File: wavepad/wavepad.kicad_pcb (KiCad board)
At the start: 2 copper layers, 18 parts, among them SW1 SW_Push, SW2 SW_Push, SW3 SW_Push, SW4 SW_Push, SW5 SW_Push, SW6 SW_Push, SW7 SW_Push, SW8 SW_Push, U1 Seeed Studio XIAO SAMD21

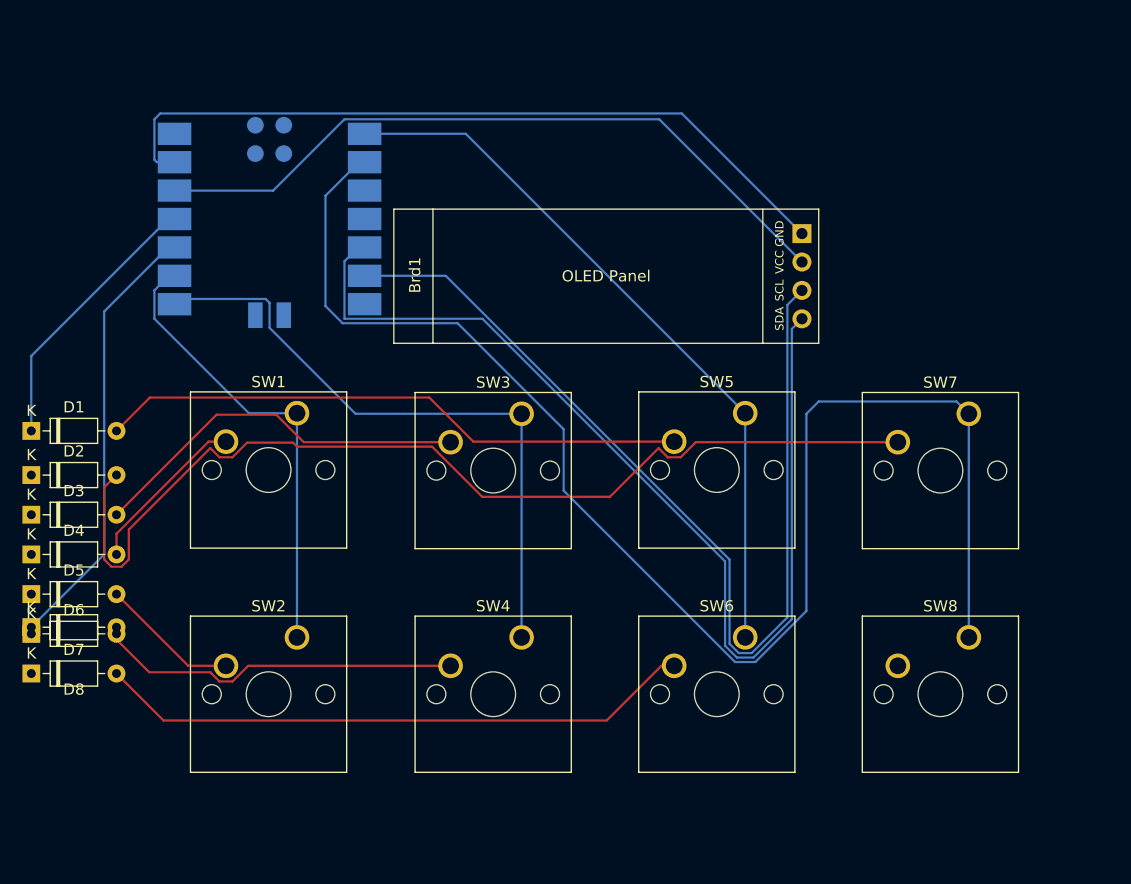
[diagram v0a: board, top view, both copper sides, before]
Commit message: actually finish design
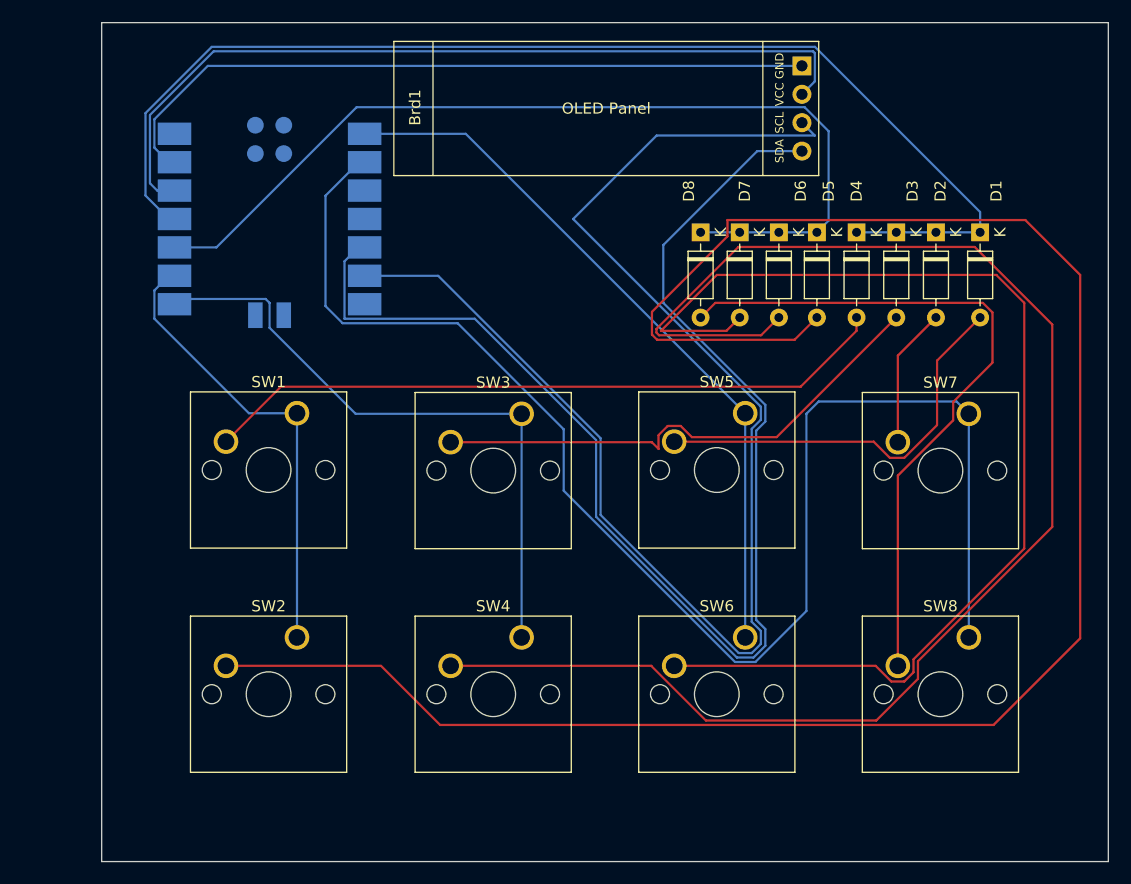
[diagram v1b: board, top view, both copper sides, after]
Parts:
- moved D1 86.7 mm to (173.6, 43.7), turned to -90 degrees
- moved D2 83.8 mm to (169.6, 43.7), turned to -90 degrees
- moved D3 81.4 mm to (166.1, 43.7), turned to -90 degrees
- moved D4 79.2 mm to (162.5, 43.7), turned to -90 degrees
- moved D5 77.4 mm to (158.9, 43.7), turned to -90 degrees
- moved D6 75.9 mm to (155.6, 43.7), turned to -90 degrees
- moved D7 74.6 mm to (152.1, 43.7), turned to -90 degrees
- moved D8 69.5 mm to (148.6, 43.7), turned to -90 degrees
- moved Brd1 15.0 mm to (121.1, 26.6)
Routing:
- net Net-(D5-A): track 12.4 -> 176.7 mm
- net Net-(D6-A): track 32.0 -> 135.4 mm
- net Row 1: track 24.6 -> 106.9 mm
- net Net-(D2-A): track 90.8 -> 12.6 mm
- net Net-(D8-A): track 0.00 -> 62.1 mm
- net Net-(D7-A): track 53.6 -> 102.6 mm
- net Net-(D4-A): track 15.1 -> 61.7 mm
- net Row 2: track 39.6 -> 84.5 mm
- net SCL: track 87.3 -> 125.7 mm
- net SDA: track 93.1 -> 118.3 mm
- net Net-(D1-A): track 52.7 -> 36.5 mm
- net Net-(D3-A): track 34.6 -> 46.5 mm
- net +3.3V: track 64.0 -> 74.6 mm
- net GND: track 68.1 -> 64.8 mm
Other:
- board outline added: 90 x 75 mm
